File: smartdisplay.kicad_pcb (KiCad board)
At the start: 2 copper layers, 100 x 40 mm, 50 parts, among them J1 Conn_01x04_Female, J2 battery, J3 FPC24/0.5MM, Q1 Q_NMOS_DSG, U1 AMS1117-3.3, U2 ESP-32S, U3 DHT11, U4 FS8205, U5 tp4056, U6 DW01

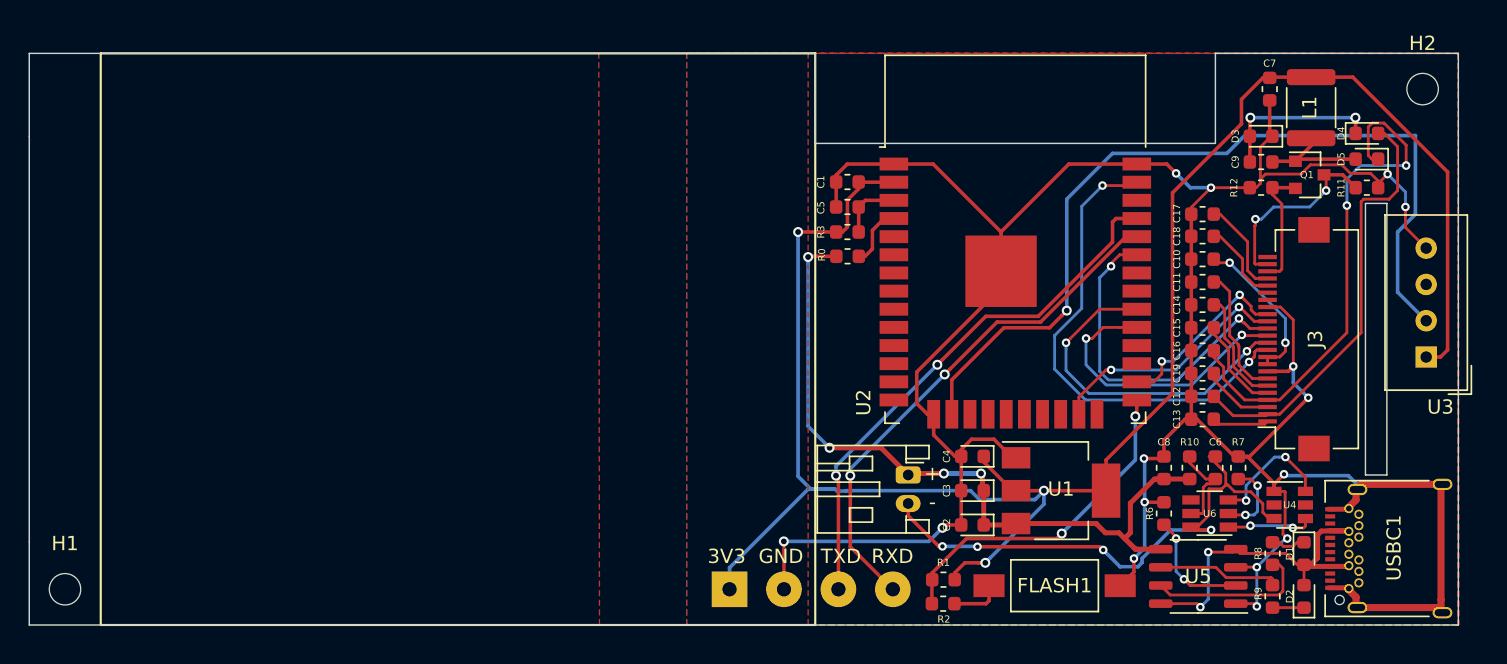
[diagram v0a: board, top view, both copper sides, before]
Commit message: finish v1.0
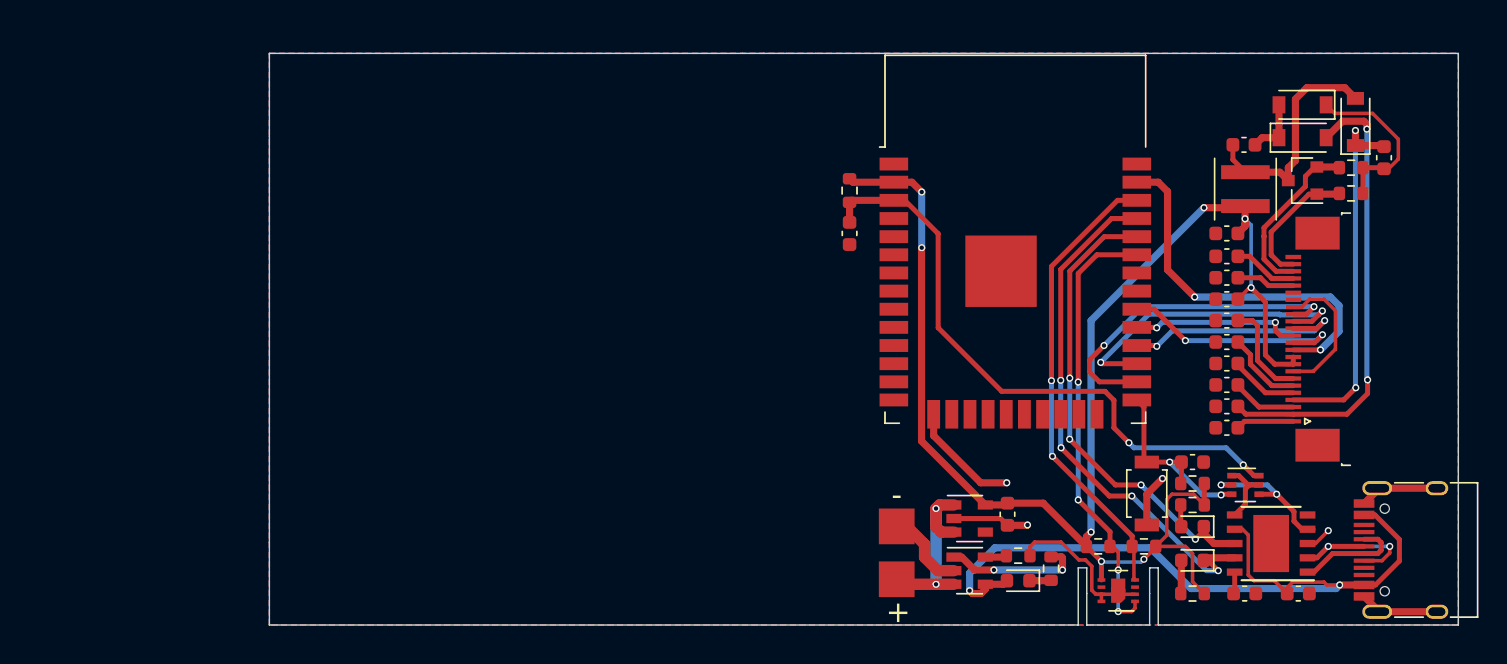
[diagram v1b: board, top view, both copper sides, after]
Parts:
- removed C18, C19: 1uF/50V, Capacitor_SMD:C_0603_1608Metric
- removed FLASH1: FLASH, Button_Switch_SMD:SW_SPST_FSMSM
- removed H1, H2: MountingHole, MountingHole:MountingHole_2.2mm_M2
- removed R0: R, Resistor_SMD:R_0603_1608Metric
- removed R11: 10K, Resistor_SMD:R_0603_1608Metric
- removed R12: 3, Resistor_SMD:R_0603_1608Metric
- removed the U4 at (188.2, 91.6)
- removed USBC1: USB_C_Plug, Connector_USB:USB_C_Receptacle_Amphenol_12401548E4-2A
- added D6: LED-red, Diode_SMD:D_0603_1608Metric, F.Cu at (169.2, 96.9)
- added R4: 10k, Resistor_SMD:R_0603_1608Metric, F.Cu at (192.5, 69.8)
- added R5: 3, Resistor_SMD:R_0603_1608Metric, F.Cu at (192.5, 68.0)
- added SW1: SW_Push, my:bt-342, F.Cu at (178.2, 90.8)
- added U2: ch340k, my:ESSOP-10_3.9x4.9mm_P1.00mm, F.Cu at (186.9, 94.3)
- added U7: TP4054, Package_TO_SOT_SMD:SOT-23-5, F.Cu at (165.8, 96.2)
- C1: value 10uF -> 1uF
- C10, C9: value 0.1uF/50V -> 1uF
- C11, C12, C13, C14, C15, C17: value 1uF/50V -> 1uF
- C16: value 1uF/50V -> 0.1uf
- C2: value 10uF -> 1uF; footprint Diode_SMD:D_0603_1608Metric -> Capacitor_SMD:C_0603_1608Metric
- C3: value 104 -> 0.1uf; footprint Diode_SMD:D_0603_1608Metric -> Capacitor_SMD:C_0603_1608Metric
- C4: value 10uF -> 4.7uF; footprint Diode_SMD:D_0603_1608Metric -> Capacitor_SMD:C_0603_1608Metric
- C5: value 104 -> 0.1uf
- C6: value C -> 1uF
- C7: value 4.7uF/50V -> 1uF
- C8: value C -> 4.7uF
- D1: value LED -> MBR0530; footprint LED_SMD:LED_0603_1608Metric -> Diode_SMD:D_SOD-123
- D2: value LED -> LED-green; footprint LED_SMD:LED_0603_1608Metric -> Diode_SMD:D_0603_1608Metric
- D3: value MBR0530 -> LED-red
- D4, D5: footprint Diode_SMD:D_0603_1608Metric -> Diode_SMD:D_SOD-123
- J1: value Conn_01x04_Female -> Conn_01x01_Female; footprint Connector_Wire:SolderWirePad_1x04_P3.81mm_Drill1mm -> my:largepoint
- J2: value battery -> USB_C_Receptacle_USB2.0; footprint Connector_JST:JST_PH_S2B-PH-K_1x02_P2.00mm_Horizontal -> Connector_USB:USB_C_Receptacle_HRO_TYPE-C-31-M-12
- J3: value FPC24/0.5MM -> Conn_01x01_Female; footprint smartdisplay:Hirose_FH12-24S-0.5SH_1x24-1MP_P0.50mm__redesign -> my:largepoint
- L1: value 68uH -> 10uH; footprint Inductor_SMD:L_1812_4532Metric -> Inductor_SMD:L_Coilcraft_XxL4040
- Q1: value Q_NMOS_DSG -> SI1308EDL
- R1, R3: value 1k -> 10k
- R10, R6, R7, R8, R9: value R -> 10k
- R2: value 470 -> 10k
- U1: value AMS1117-3.3 -> DDC114TU-7-F; footprint Package_TO_SOT_SMD:SOT-223-3_TabPin2 -> Package_TO_SOT_SMD:SOT-363_SC-70-6
- U3: value DHT11 -> 24pinconnecter; footprint Sensor:Aosong_DHT11_5.5x12.0_P2.54mm -> my:epd-24pin
- U5: value tp4056 -> SHT31-DIS; footprint Package_SO:SOP-8_3.9x4.9mm_P1.27mm -> Sensor_Humidity:Sensirion_DFN-8-1EP_2.5x2.5mm_P0.5mm_EP1.1x1.7mm
- U6: value DW01 -> ME6211C33M5G-N; footprint Package_TO_SOT_SMD:TSOT-23-6 -> Package_TO_SOT_SMD:SOT-23-5
- moved C5 41.6 mm to (188.8, 97.8), turned to 0 degrees
- moved J2 36.3 mm to (197.4, 94.8), turned to 90 degrees
- moved J3 30.7 mm to (160.7, 93.1), turned to 0 degrees
- moved C6 30.4 mm to (157.4, 72.6), turned to 270 degrees
- moved D1 29.1 mm to (189.1, 65.9), turned to 0 degrees
- moved C4 28.9 mm to (185.0, 66.4)
- moved D3 27.7 mm to (181.4, 93.1)
- moved C1 27.1 mm to (183.8, 74.2)
- moved C17 25.0 mm to (168.4, 92.2), turned to 270 degrees
- moved C2 24.8 mm to (183.8, 75.7)
- moved C3 20.4 mm to (185.1, 97.8)
- moved R2 18.8 mm to (181.4, 91.6)
- moved R1 17.5 mm to (181.4, 97.8), turned to 180 degrees
- moved C8 17.0 mm to (183.8, 72.6), turned to 0 degrees
- moved U6 16.8 mm to (165.8, 92.5), turned to 0 degrees
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- renumbered U2 to U4
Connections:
- C1 pad 1: /VDD3V3 -> Net-(C1-Pad1)
- C10 pad 1: /VDD3.3V -> Net-(C10-Pad1)
- C12 pad 1: /PREVGL -> Net-(C12-Pad1)
- C14 pad 1: Net-(C14-Pad1) -> PREVGL
- C16 pad 1: /PREVGH -> GND
- C16 pad 2: GND -> IO0
- C17 pad 1: Net-(C17-Pad1) -> +3V3
- C2 pad 1: /B+ -> Net-(C2-Pad1)
- C3 pad 1: /B+ -> GND
- C3 pad 2: GND -> Net-(C3-Pad2)
- C4 pad 1: /VDD3V3 -> Net-(C4-Pad1)
- C4 pad 2: GND -> Net-(C4-Pad2)
- C5 pad 1: /EN -> +5V
- C6 pad 1: Net-(C6-Pad1) -> EN
- C6 pad 2: /B- -> GND
- C7 pad 1: GND -> +3V3
- C7 pad 2: /VDD3V3 -> GND
- C8 pad 1: /B+ -> GND
- C8 pad 2: GND -> +3V3
- C9 pad 1: Net-(C9-Pad1) -> PREVGH
- C9 pad 2: Net-(C9-Pad2) -> GND
- D1 pad 1: Net-(D1-Pad1) -> Net-(C4-Pad1)
- D1 pad 2: /USB5V -> PREVGL
- D2 pad 1: Net-(D2-Pad1) -> RX
- D2 pad 2: /USB5V -> Net-(D2-Pad2)
- D3 pad 1: GND -> TX
- D3 pad 2: Net-(C9-Pad1) -> Net-(D3-Pad2)
- D4 pad 1: Net-(C9-Pad1) -> GND
- D4 pad 2: /PREVGL -> Net-(C4-Pad1)
- D5 pad 1: /PREVGH -> PREVGH
- D5 pad 2: Net-(C9-Pad2) -> Net-(C4-Pad2)
- J1 pad 1: /VDD3V3 -> BAT+
- J3 pad 1: Net-(J3-Pad1) -> GND
- L1 pad 1: /VDD3V3 -> +3V3
- L1 pad 2: Net-(C9-Pad2) -> Net-(C4-Pad2)
- Q1 pad 1: Net-(C9-Pad2) -> GDR
- Q1 pad 2: /RESE -> RESE
- Q1 pad 3: /GDR -> Net-(C4-Pad2)
- R1 pad 1: /IO0 -> +3V3
- R1 pad 2: /VDD3V3 -> Net-(D2-Pad2)
- R10 pad 1: /B+ -> Net-(R10-Pad1)
- R10 pad 2: Net-(C6-Pad1) -> GND
- R2 pad 1: Net-(FLASH1-Pad1) -> +3V3
- R2 pad 2: /IO0 -> Net-(D3-Pad2)
- R3 pad 1: /EN -> +3V3
- R3 pad 2: /VDD3V3 -> EN
- R6 pad 1: Net-(R6-Pad1) -> +3V3
- R6 pad 2: GND -> IO0
- R7 pad 1: Net-(R7-Pad1) -> +3V3
- R7 pad 2: GND -> SDA
- R8 pad 1: Net-(R8-Pad1) -> +3V3
- R8 pad 2: Net-(D1-Pad1) -> SCL
- R9 pad 1: Net-(R9-Pad1) -> Net-(D6-Pad1)
- R9 pad 2: Net-(D2-Pad1) -> Net-(R9-Pad2)
- U1 pad 1: GND -> RTS
- U1 pad 2: /VDD3V3 -> DTR
- U1 pad 3: /B+ -> IO0
- U3 pad 1: /VDD3V3 -> (no net)
- U3 pad 2: /IO16 -> GDR
- U3 pad 3: Net-(U3-Pad3) -> RESE
- U3 pad 4: GND -> Net-(C1-Pad1)
- U4 pad 10: Net-(U2-Pad10) -> (no net)
- U4 pad 11: Net-(U2-Pad11) -> (no net)
- U4 pad 12: Net-(U2-Pad12) -> (no net)
- U4 pad 13: Net-(U2-Pad13) -> (no net)
- U4 pad 14: Net-(U2-Pad14) -> (no net)
- U4 pad 16: /IO16 -> (no net)
- U4 pad 17: Net-(U2-Pad17) -> (no net)
- U4 pad 18: Net-(U2-Pad18) -> (no net)
- U4 pad 19: Net-(U2-Pad19) -> (no net)
- U4 pad 2: /VDD3V3 -> +3V3
- U4 pad 20: Net-(U2-Pad20) -> (no net)
- U4 pad 21: Net-(U2-Pad21) -> (no net)
- U4 pad 22: Net-(U2-Pad22) -> (no net)
- U4 pad 23: /REST -> (no net)
- U4 pad 24: /IO2 -> (no net)
- U4 pad 25: /IO0 -> IO0
- U4 pad 26: /BUSY -> BUSY
- U4 pad 27: Net-(U2-Pad27) -> REST
- U4 pad 28: Net-(U2-Pad28) -> DC
- U4 pad 29: /CS -> CS
- U4 pad 3: /EN -> EN
- U4 pad 30: /CLK -> SCLK
- U4 pad 31: Net-(U2-Pad31) -> (no net)
- U4 pad 32: Net-(U2-Pad32) -> (no net)
- U4 pad 33: /DC -> SDA
- U4 pad 34: /RX -> TX
- U4 pad 35: /TX -> RX
- U4 pad 36: Net-(U2-Pad36) -> SCL
- U4 pad 37: /DIN -> DIN
- U4 pad 4: Net-(R0-Pad1) -> (no net)
- U4 pad 5: Net-(U2-Pad5) -> (no net)
- U4 pad 6: Net-(U2-Pad6) -> (no net)
- U4 pad 7: Net-(U2-Pad7) -> (no net)
- U4 pad 8: Net-(U2-Pad8) -> (no net)
- U4 pad 9: Net-(U2-Pad9) -> (no net)
- U5 pad 1: GND -> SDA
- U5 pad 2: Net-(R6-Pad1) -> GND
- U5 pad 3: GND -> (no net)
- U5 pad 4: /USB5V -> SCL
- U5 pad 5: /B+ -> +3V3
- U5 pad 6: Net-(R9-Pad1) -> (no net)
- U5 pad 7: Net-(R8-Pad1) -> GND
- U5 pad 8: /USB5V -> GND
- U6 pad 1: /OD -> BAT+
- U6 pad 2: Net-(R7-Pad1) -> GND
- U6 pad 3: /OC -> BAT+
- U6 pad 4: Net-(U6-Pad4) -> (no net)
- U6 pad 5: Net-(C6-Pad1) -> +3V3
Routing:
- net GND: track 211.9 -> 70.2 mm, vias 15 -> 4
- net /VDD3V3: track 138.7 -> 0.00 mm, vias 3 -> 0
- net +3V3: track 0.00 -> 105.4 mm, vias 0 -> 8
- net /IO16: track 60.8 -> 0.00 mm, vias 1 -> 0
- net /B+: track 59.6 -> 0.00 mm, vias 4 -> 0
- net +5V: track 0.00 -> 53.5 mm, vias 0 -> 2
- net EN: track 0.00 -> 43.1 mm, vias 0 -> 2
- net /B-: track 38.6 -> 0.00 mm, vias 4 -> 0
- net /TX: track 37.7 -> 0.00 mm, vias 2 -> 0
- net RX: track 0.00 -> 37.4 mm, vias 0 -> 4
- net /RX: track 36.4 -> 0.00 mm, vias 2 -> 0
- net /PREVGH: track 36.4 -> 0.00 mm, vias 2 -> 0
- net /DIN: track 34.2 -> 0.00 mm, vias 2 -> 0
- net TX: track 0.00 -> 33.2 mm, vias 0 -> 4
- net SCL: track 0.00 -> 32.3 mm, vias 0 -> 2
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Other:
- board size 100 x 40 mm -> 83.2 x 40 mm
- board text added: "BLab"
- board text added: "smartdisplay"
- board text removed: "3V3"
- board text removed: "BLab_SmartDisplay"
- board text removed: "GND"
- board text removed: "RXD"
- board text removed: "TXD"
